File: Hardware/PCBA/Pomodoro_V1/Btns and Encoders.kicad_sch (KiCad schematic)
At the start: 0 parts

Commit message: Implemented the Rotary encoder, the buttons, the IMU, Added it to the PCB (All the space constraining elements are now placed)
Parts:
- added C22, C26, C27: 100n, symbol Device:C
- added R10, R11, R12, R5, R6, R7, R9: 4k7, symbol Device:R
- added S1: PEC12R-2220F-S0024, Rotary_Encoder:PEC12R-2220F-S0024, symbol PEC12R-2220F-S0024:PEC12R-2220F-S0024
- added SW1: SW_Push, symbol Switch:SW_Push
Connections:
- new net: R5.2, R6.1, SW1.2
- new net: R11.2, R9.2, S1.A (CHANNEL_A)
- new net: R10.2, R12.2, S1.B (CHANNEL_B)
- new net +3V3: R10.1, R5.1, R7.1, R9.1
- new net GND: C22.2, C26.2, C27.2, S1.2, S1.C (COMMON), S1.S1 (SHIELD), S1.S2 (SHIELD), SW1.1
- new net GPIO_IN (Encoder BTN): R7.2, S1.1
- new net GPIO_IN (Trigger Btn): C22.1, R6.2
- new net TIM2_CH1 (Encoder Dial): C27.1, R11.1
- new net TIM2_CH2 (Encoder Dial): C26.1, R12.1
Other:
- note added: "Rotary Encoder with Button"
- note added: "Trigger Button (Cherry Mx)"

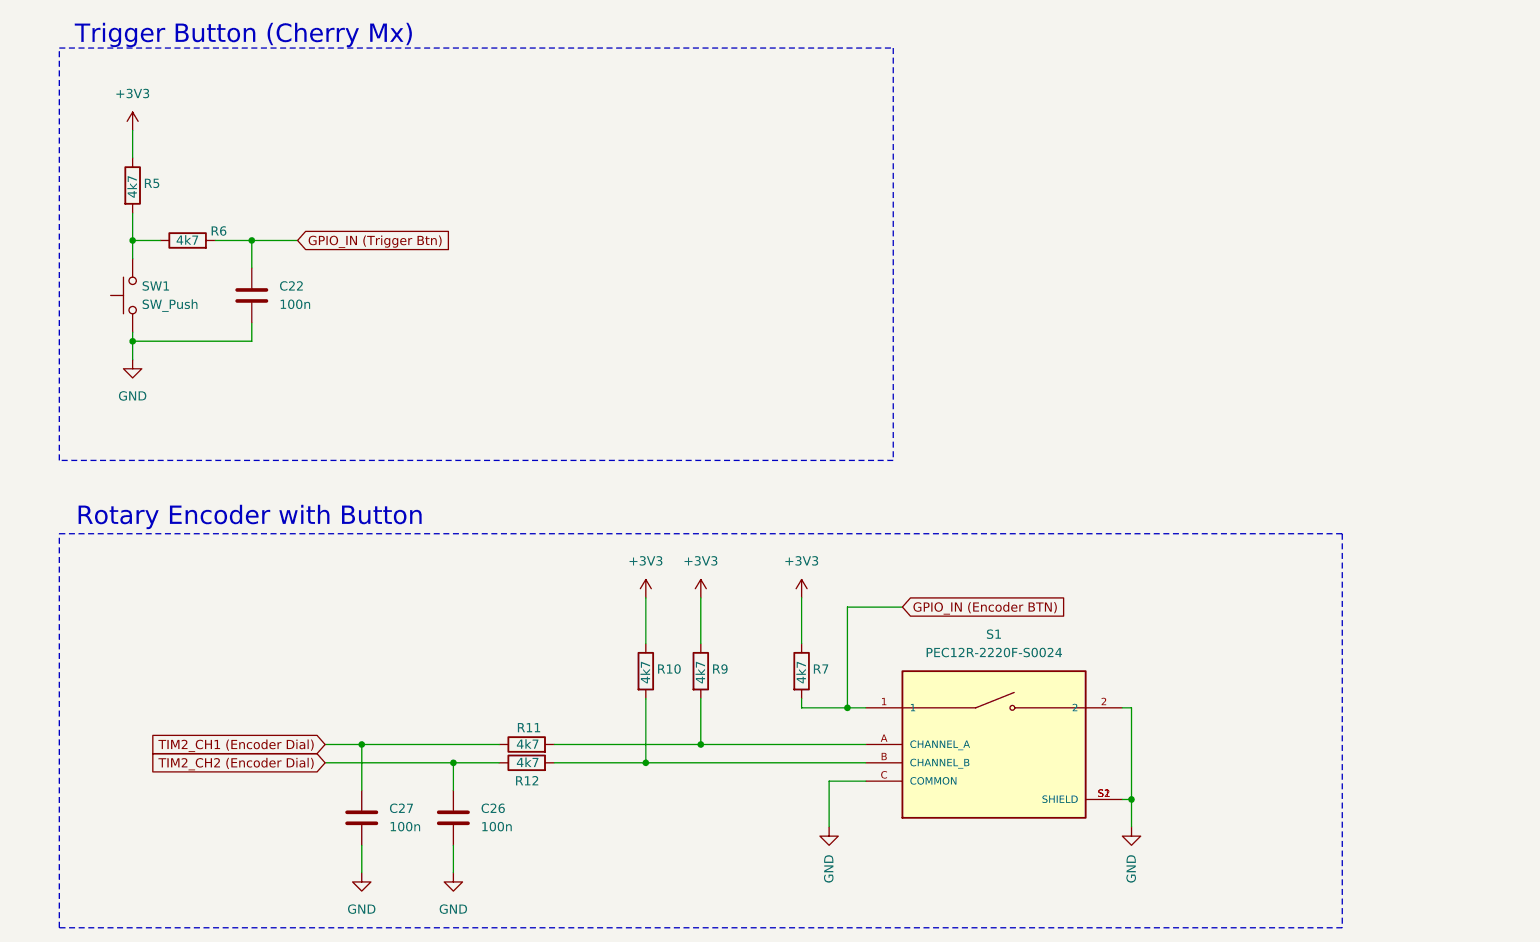
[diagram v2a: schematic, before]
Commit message: Finalized the schematic, First Draft of the finished Layout
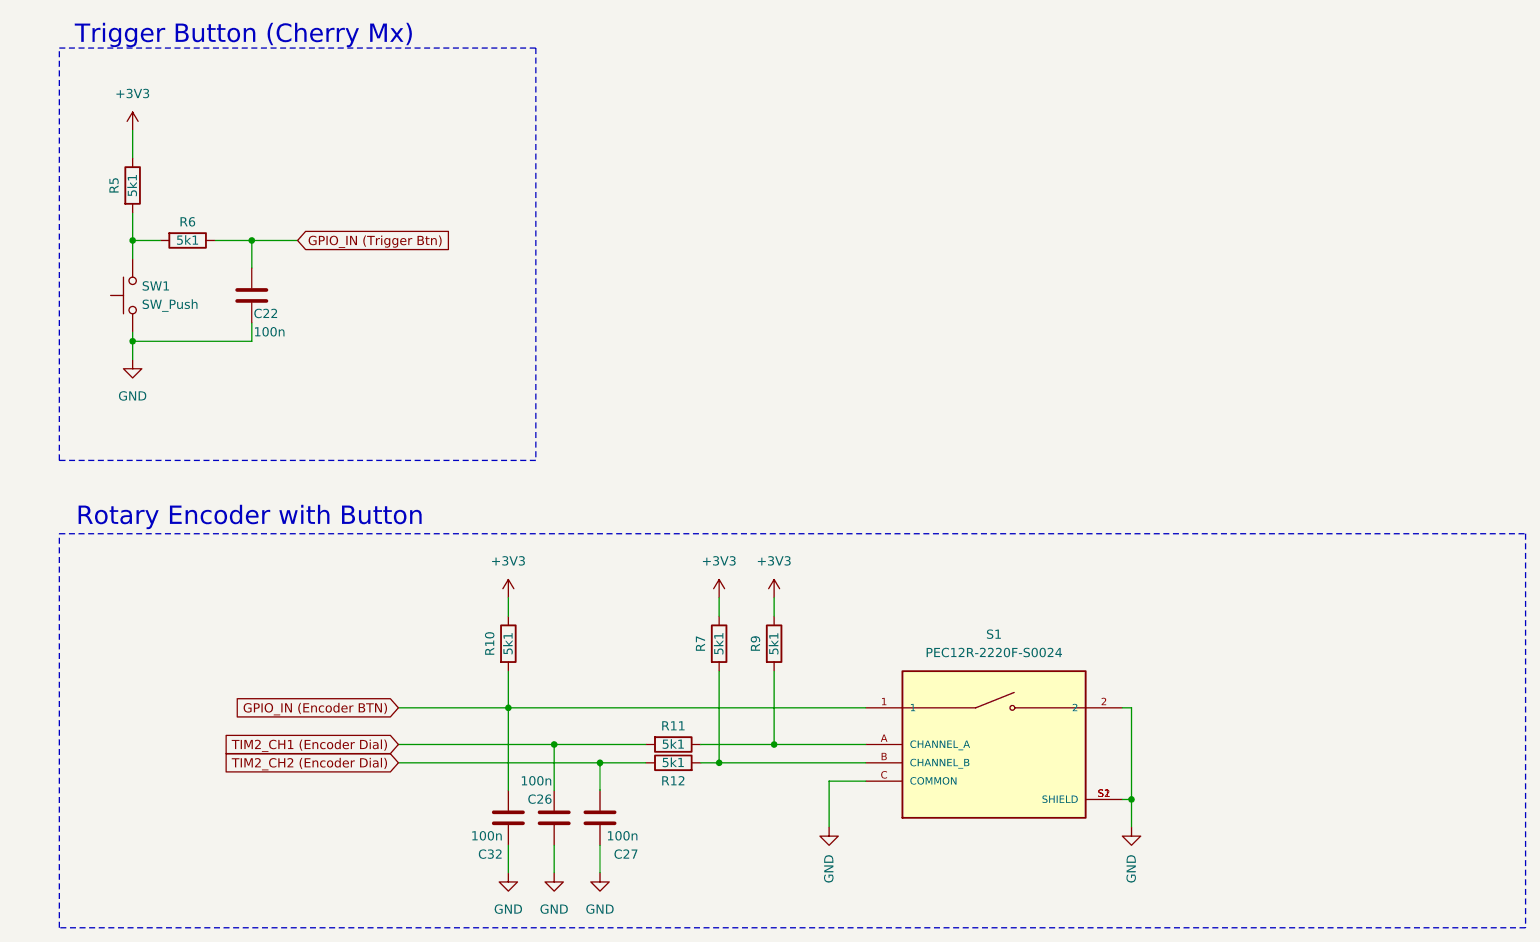
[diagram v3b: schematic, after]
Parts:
- added C32: 100n, Capacitor_SMD:C_0805_2012Metric, symbol Device:C
- C22, C26, C27: footprint (none) -> Capacitor_SMD:C_0805_2012Metric
- R10, R11, R12, R5, R6, R7, R9: value 4k7 -> 5k1; footprint (none) -> Resistor_SMD:R_0805_2012Metric; Part ID (none) -> CR0805-FX-5101ELF
- SW1: footprint (none) -> Button_Switch_Keyboard:SW_Cherry_MX_1.00u_PCB
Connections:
- net GND: now also C26.1, C27.1, C32.1; no longer C26.2, C27.2
- net GPIO_IN (Encoder BTN): now also R10.2, C32.2; no longer R7.2
- net GPIO_IN (Trigger Btn): now also R6.1; no longer R6.2
- net TIM2_CH1 (Encoder Dial): now also C26.2, R11.2; no longer C27.1, R11.1
- net TIM2_CH2 (Encoder Dial): now also C27.2; no longer C26.1
- net at R5.2, SW1.2: now also R6.2; no longer R6.1
- net at R9.2, S1.A (CHANNEL_A): now also R11.1; no longer R11.2
- net at R12.2, S1.B (CHANNEL_B): now also R7.2; no longer R10.2
